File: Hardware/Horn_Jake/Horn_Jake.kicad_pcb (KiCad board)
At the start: 2 copper layers, 21 parts, among them J1 Horn 1, J2 Horn 2, J3 Horn Control, J4 Power, Q1 N-type transistor, SW1 Debug Switch

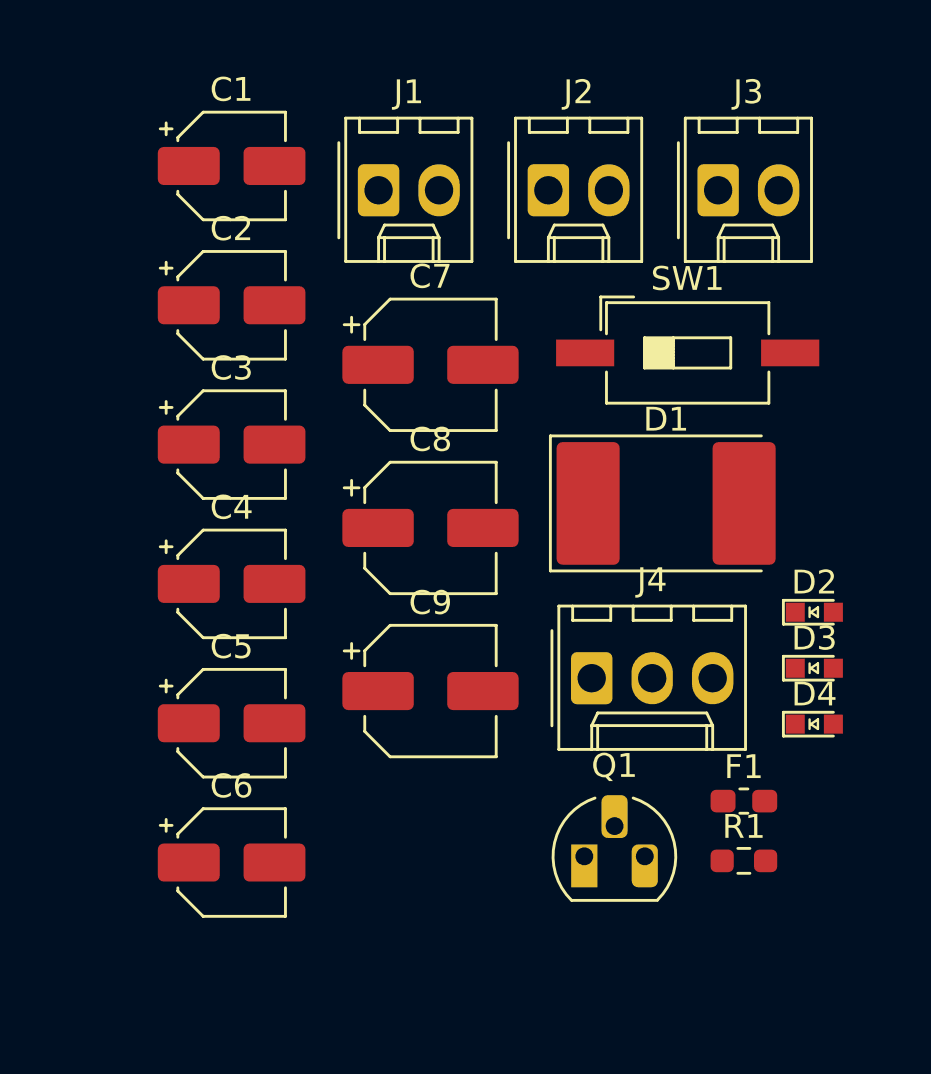
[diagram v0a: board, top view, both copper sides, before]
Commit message: Hardware Advanced Project Completion
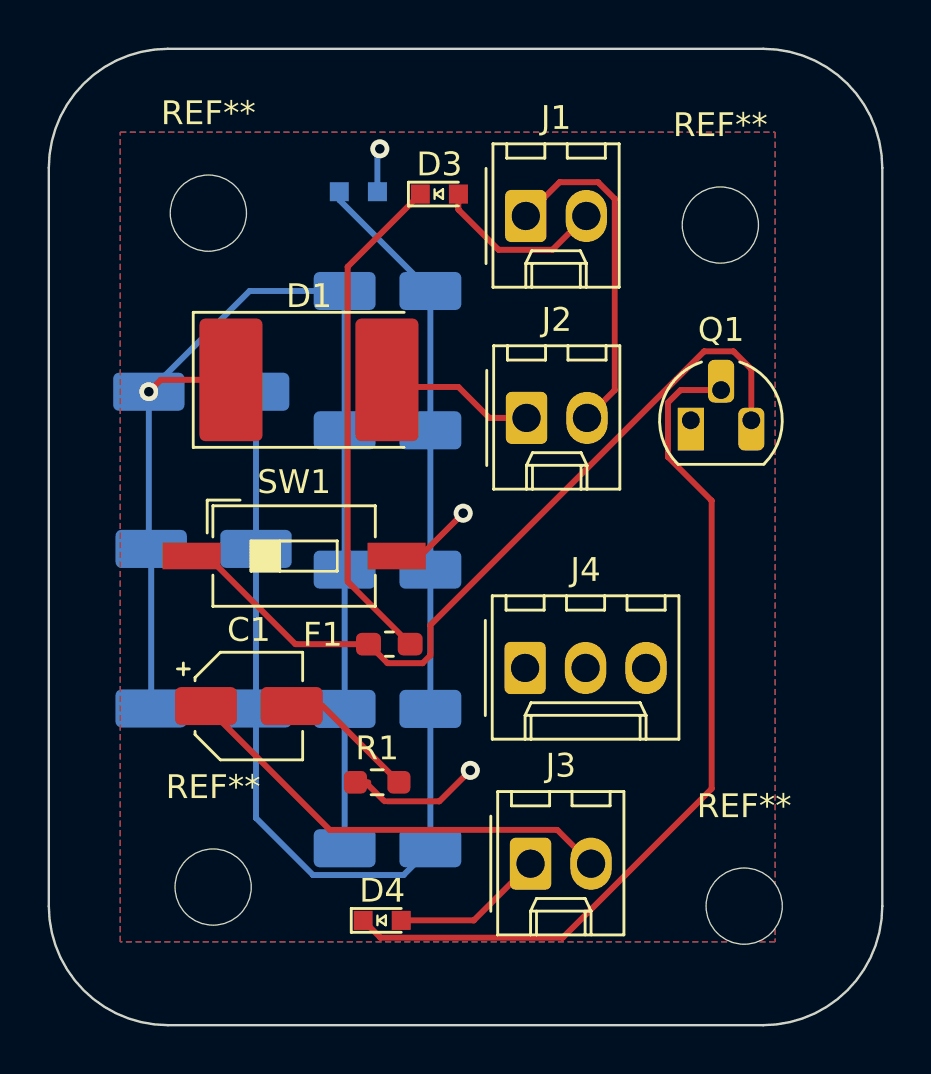
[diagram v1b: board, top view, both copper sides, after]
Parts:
- added REF**: MountingHole_3.2mm_M3, MountingHole:MountingHole_3.2mm_M3, F.Cu at (116.9, 97.2)
- added REF**: MountingHole_3.2mm_M3, MountingHole:MountingHole_3.2mm_M3, F.Cu at (138.2, 69.4)
- added REF**: MountingHole_3.2mm_M3, MountingHole:MountingHole_3.2mm_M3, F.Cu at (139.2, 98.0)
- added REF**: MountingHole_3.2mm_M3, MountingHole:MountingHole_3.2mm_M3, F.Cu at (116.7, 68.9)
- C2, C3, C4, C5, C6, C7, C8, C9, D2: moved to B.Cu
- moved J3 29.4 mm to (130.2, 96.2)
- moved D2 26.0 mm to (123.0, 68.0)
- moved D3 25.4 mm to (126.4, 68.1)
- moved C1 22.7 mm to (118.4, 89.6)
- moved D4 19.9 mm to (124.0, 98.6)
- moved Q1 18.8 mm to (137.0, 77.6)
- moved SW1 18.6 mm to (120.3, 83.3)
- moved F1 16.3 mm to (124.3, 87.0)
- moved D1 15.9 mm to (120.9, 75.9)
- moved R1 15.7 mm to (123.8, 92.8)
- moved C7 9.69 mm to (116.4, 76.4), turned to 180 degrees
- moved J2 9.60 mm to (130.1, 77.5)
- moved C8 9.57 mm to (116.5, 83.0), turned to 180 degrees
- moved C9 9.56 mm to (116.5, 89.7), turned to 180 degrees
- moved C3 6.57 mm to (124.2, 78.0), turned to 180 degrees
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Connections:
- C2 pad 1: +24V -> Net-(D2-K)
- C3 pad 1: +24V -> Net-(D2-K)
- C4 pad 1: +24V -> Net-(D2-K)
- C5 pad 1: +24V -> Net-(D2-K)
- C6 pad 1: +24V -> Net-(D2-K)
- C7 pad 1: +24V -> Net-(D2-K)
- C8 pad 1: +24V -> Net-(D2-K)
- C9 pad 1: +24V -> Net-(D2-K)
- D2 pad 1: +24V -> Net-(D2-K)
- D2 pad 2: Net-(D2-A) -> +24V
- J4 pad 2: Net-(D2-A) -> +24V
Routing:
- net Net-(D2-K): track 0.00 -> 55.9 mm
- net Net-(D1-K): track 0.00 -> 50.4 mm, vias 0 -> 1
- net /HORN_CTL: track 0.00 -> 36.9 mm
- net Net-(Q1-B1): track 0.00 -> 34.0 mm
- net Net-(D3-K): track 0.00 -> 21.3 mm
- net Net-(J3-Pin_2): track 0.00 -> 18.9 mm
- net Net-(J1-Pin_1): track 0.00 -> 14.3 mm
- net GND: track 0.00 -> 9.24 mm, vias 0 -> 2
- net /HORN_IN: track 0.00 -> 7.31 mm
- net Net-(D1-A): track 0.00 -> 6.52 mm
- net Net-(D4-A): track 0.00 -> 6.42 mm
- net Net-(C1-Pad2): track 0.00 -> 5.83 mm
- net +24V: track 0.00 -> 1.94 mm, vias 0 -> 1
- added copper zone on F.Cu, net +24V
- added copper zone on B.Cu, net GND
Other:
- board outline added: 35 x 41 mm
